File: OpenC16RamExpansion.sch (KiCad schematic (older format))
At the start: 4 parts, among them U1 74LS257, U2 74LS257, U3 4464, U4 4464

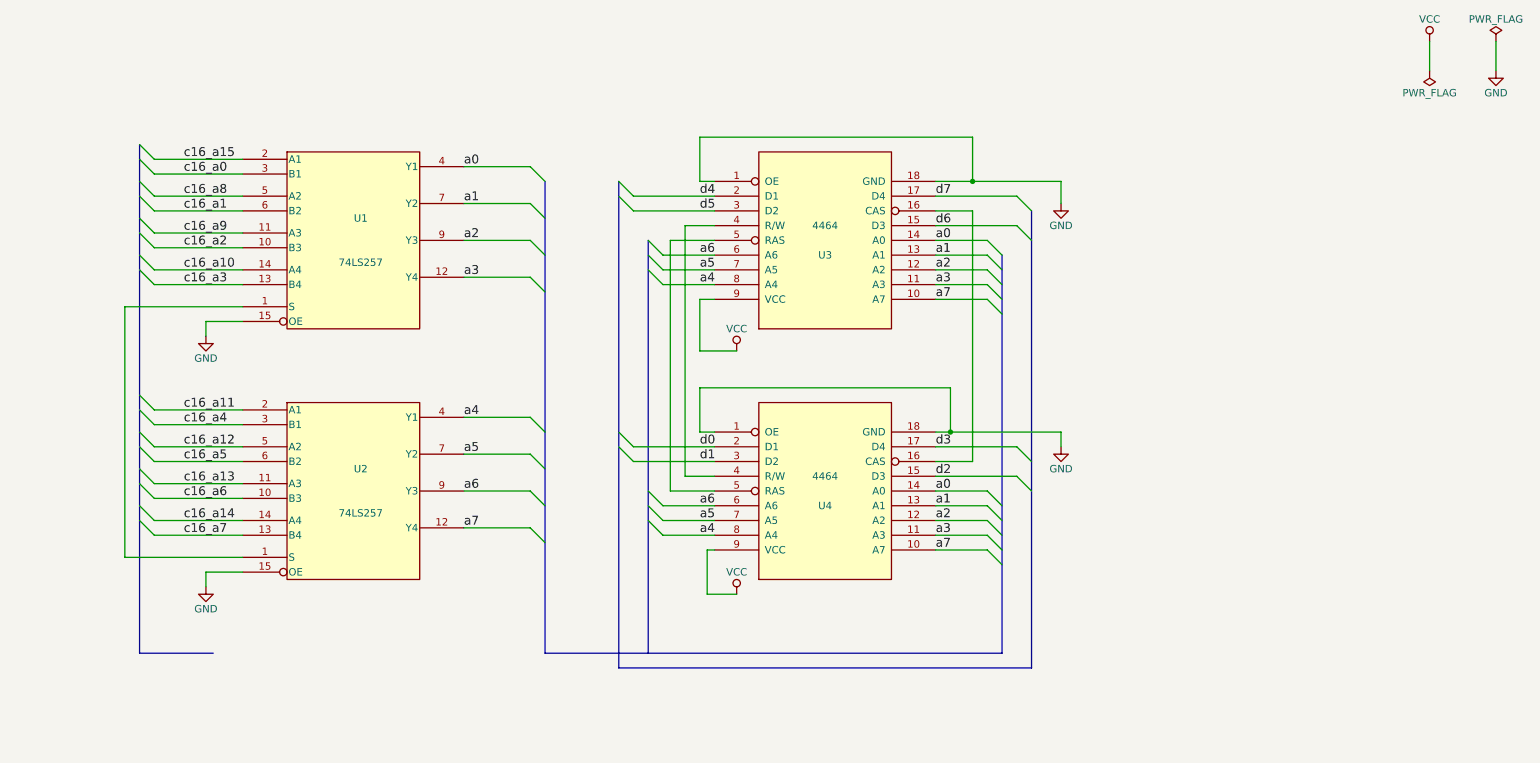
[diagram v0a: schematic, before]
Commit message: Complete schematics
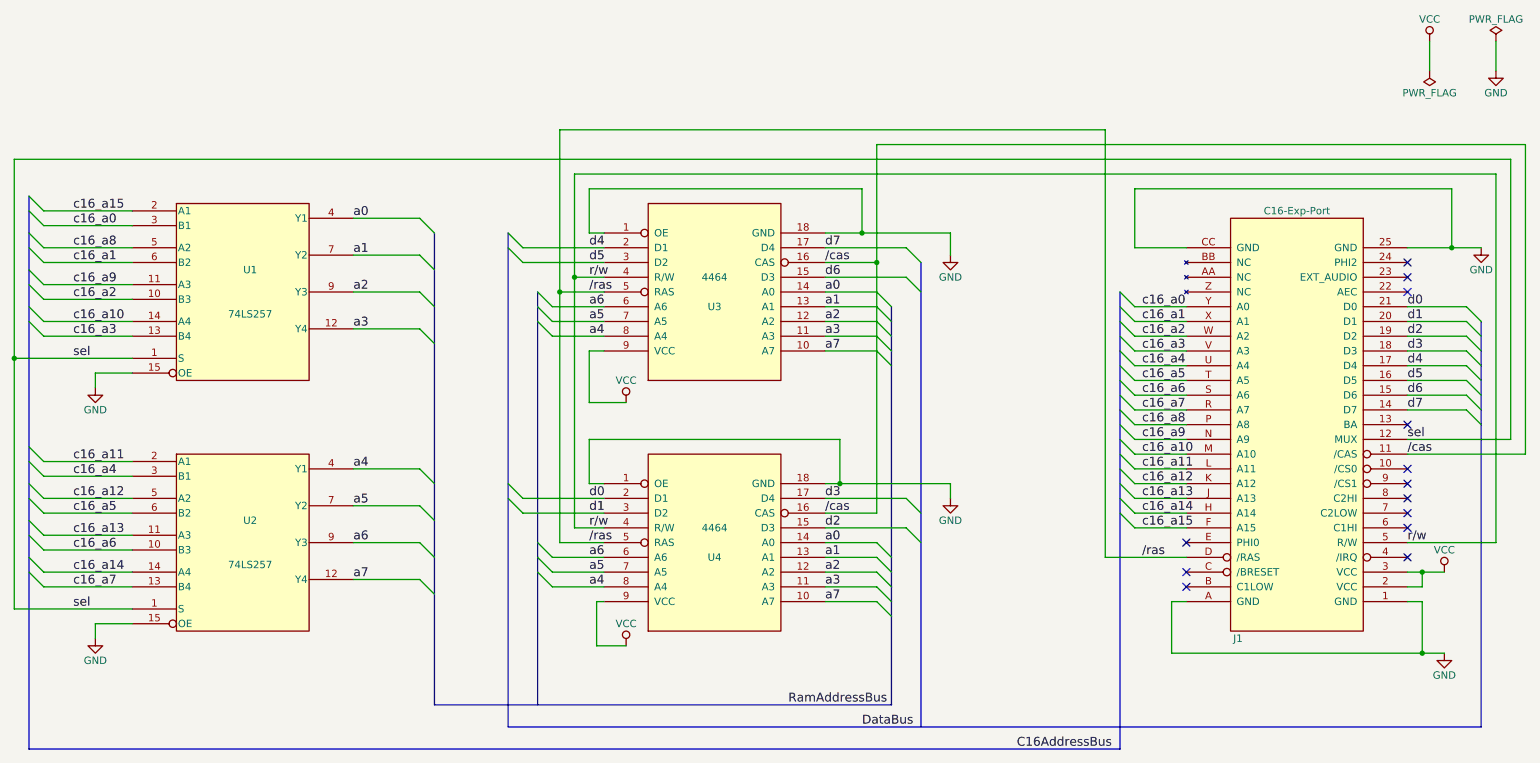
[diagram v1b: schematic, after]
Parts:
- added J1: C16-Exp-Port, C16_Cart_Conn:C16_Cart_Conn, symbol C16-Exp-Port
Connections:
- net GND: now also J1.1 (GND), J1.25 (GND), J1.A (GND), J1.CC (GND)
- net VCC: now also J1.2 (VCC), J1.3 (VCC)
- net c16_a0: now also J1.Y (A0)
- net c16_a1: now also J1.X (A1)
- net c16_a10: now also J1.M (A10)
- net c16_a11: now also J1.L (A11)
- net c16_a12: now also J1.K (A12)
- net c16_a13: now also J1.J (A13)
- net c16_a14: now also J1.H (A14)
- net c16_a15: now also J1.F (A15)
- net c16_a2: now also J1.W (A2)
- net c16_a3: now also J1.V (A3)
- net c16_a4: now also J1.U (A4)
- net c16_a5: now also J1.T (A5)
- net c16_a6: now also J1.S (A6)
- net c16_a7: now also J1.R (A7)
- net c16_a8: now also J1.P (A8)
- net c16_a9: now also J1.N (A9)
- net d0: now also J1.21 (D0)
- net d1: now also J1.20 (D1)
- net d2: now also J1.19 (D2)
- net d3: now also J1.18 (D3)
- net d4: now also J1.17 (D4)
- net d5: now also J1.16 (D5)
- net d6: now also J1.15 (D6)
- net d7: now also J1.14 (D7)
- net sel: now reaches U1.1 (S), U2.1 (S)
- net sel: now also J1.12 (MUX)
- net /cas: now reaches U3.16 (CAS), U4.16 (CAS)
- net /cas: now also J1.11 (/CAS)
- net r/w: now reaches U3.4 (R/W), U4.4 (R/W)
- net r/w: now also J1.5 (R/W)
- net /ras: now reaches U3.5 (RAS), U4.5 (RAS)
- net /ras: now also J1.D (/RAS)
- no-connect marks 0 -> 13
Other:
- moved on the sheet: U1, U2, U3, U4

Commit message: Almost there...
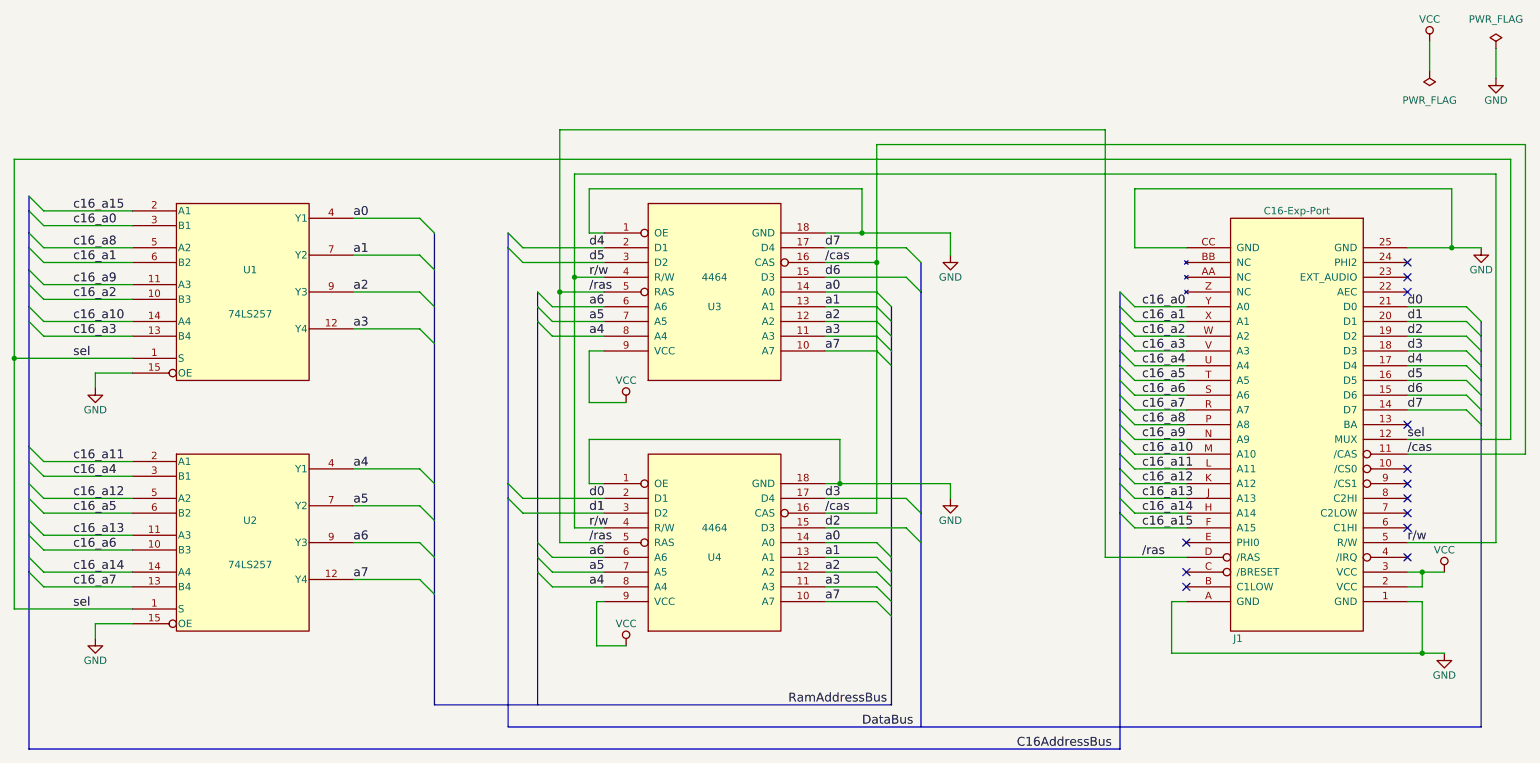
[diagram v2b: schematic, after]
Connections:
- net a0 is gone; now on net /cas: U1.4 (Y1), U3.14 (A0), U4.14 (A0)
- net a1 is gone; now on net /cas: U1.7 (Y2), U3.13 (A1), U4.13 (A1)
- net a2 is gone; now on net /cas: U1.9 (Y3), U3.12 (A2), U4.12 (A2)
- net a3 is gone; now on net /cas: U1.12 (Y4), U3.11 (A3), U4.11 (A3)
- net a7 is gone; now on net /cas: U2.12 (Y4), U3.10 (A7), U4.10 (A7)
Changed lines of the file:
@@
 L GND #PWR06
 U 1 1 598EC57B
-P 10750 1050
-F 0 "#PWR06" H 10750 800 50  0001 C CNN
-F 1 "GND" H 10750 900 50  0000 C CNN
-F 2 "" H 10750 1050 50  0001 C CNN
-F 3 "" H 10750 1050 50  0001 C CNN
-	1    10750 1050
+P 10750 1100
+F 0 "#PWR06" H 10750 850 50  0001 C CNN
+F 1 "GND" H 10750 950 50  0000 C CNN
+F 2 "" H 10750 1100 50  0001 C CNN
+F 3 "" H 10750 1100 50  0001 C CNN
+	1    10750 1100
 	1    0    0    -1
 $EndComp
@@
 L PWR_FLAG #FLG07
 U 1 1 598EC590
-P 10750 850
-F 0 "#FLG07" H 10750 925 50  0001 C CNN
-F 1 "PWR_FLAG" H 10750 1000 50  0000 C CNN
-F 2 "" H 10750 850 50  0001 C CNN
-F 3 "" H 10750 850 50  0001 C CNN
-	1    10750 850
+P 10750 900
+F 0 "#FLG07" H 10750 975 50  0001 C CNN
+F 1 "PWR_FLAG" H 10750 1100 50  0000 C CNN
+F 2 "" H 10750 900 50  0001 C CNN
+F 3 "" H 10750 900 50  0001 C CNN
+	1    10750 900
 	1    0    0    -1
 $EndComp
@@
 P 10300 1050
 F 0 "#FLG08" H 10300 1125 50  0001 C CNN
-F 1 "PWR_FLAG" H 10300 1200 50  0000 C CNN
+F 1 "PWR_FLAG" H 10300 1250 50  0000 C CNN
 F 2 "" H 10300 1050 50  0001 C CNN
 F 3 "" H 10300 1050 50  0001 C CNN
@@
 NoConn ~ 10150 4350
 Wire Wire Line
-	6200 2150 7050 2150
+	6200 2150 6450 2150
+Wire Wire Line
+	6450 2150 7050 2150
 Wire Wire Line
 	7050 2150 7050 2300
@@
 	7050 3850 7050 3950
 Wire Wire Line
-	6200 3850 7050 3850
+	6200 3850 6300 3850
+Wire Wire Line
+	6300 3850 7050 3850
 Wire Wire Line
 	4850 4950 4650 4950
@@
 	10300 850  10300 1050
 Wire Wire Line
-	10750 1050 10750 850
+	10750 1100 10750 900
 Wire Wire Line
 	6550 4050 6200 4050
 Wire Wire Line
-	6550 1550 6550 4050
+	6550 1550 6550 2350
+Wire Wire Line
+	6550 2350 6550 2550
+Wire Wire Line
+	6550 2550 6550 2650
+Wire Wire Line
+	6550 2650 6550 2750
+Wire Wire Line
+	6550 2750 6550 2850
+Wire Wire Line
+	6550 2850 6550 2950
+Wire Wire Line
+	6550 2950 6550 4050
 Wire Wire Line
 	6550 2350 6200 2350
@@
 	6200 4650 6550 4650
 Wire Bus Line
-	6650 2650 6650 5350
+	6650 2650 6650 2750
+Wire Bus Line
+	6650 2750 6650 2850
+Wire Bus Line
+	6650 2850 6650 2950
+Wire Bus Line
+	6650 2950 6650 3050
+Wire Bus Line
+	6650 3050 6650 4350
+Wire Bus Line
+	6650 4350 6650 4450
+Wire Bus Line
+	6650 4450 6650 4550
+Wire Bus Line
+	6650 4550 6650 4650
+Wire Bus Line
+	6650 4650 6650 4750
+Wire Bus Line
+	6650 4750 6650 5350
 Wire Wire Line
 	4400 4250 4700 4250
 Wire Wire Line
-	4400 1450 4400 4250
+	4400 1450 4400 2550
+Wire Wire Line
+	4400 2550 4400 4250
 Wire Wire Line
 	4400 2550 4700 2550
@@
 	4700 4550 4350 4550
 Wire Bus Line
-	4250 2550 4250 5350
+	4250 2550 4250 2650
+Wire Bus Line
+	4250 2650 4250 2750
+Wire Bus Line
+	4250 2750 4250 4250
+Wire Bus Line
+	4250 4250 4250 4350
+Wire Bus Line
+	4250 4350 4250 4450
+Wire Bus Line
+	4250 4450 4250 5350
 Wire Wire Line
 	1500 3100 1250 3100
@@
 	1500 3000 700  3000
 Wire Wire Line
-	700  1650 700  4700
+	700  1650 700  3000
+Wire Wire Line
+	700  3000 700  4700
 Wire Wire Line
 	700  4700 1500 4700
@@
 	6200 4150 6750 4150
 Wire Bus Line
-	6850 2350 6850 5500
+	6850 2350 6850 2550
+Wire Bus Line
+	6850 2550 6850 4050
+Wire Bus Line
+	6850 4050 6850 4250
+Wire Bus Line
+	6850 4250 6850 5500
 Wire Bus Line
 	10650 5500 4050 5500
@@
 	4700 4050 4150 4050
 Wire Bus Line
-	4050 5500 4050 2150
+	4050 5500 4050 3950
+Wire Bus Line
+	4050 3950 4050 3850
+Wire Bus Line
+	4050 3850 4050 2250
+Wire Bus Line
+	4050 2250 4050 2150
 Wire Wire Line
 	4500 4150 4700 4150
 Wire Wire Line
-	4500 1750 4500 4150
+	4500 1750 4500 2450
+Wire Wire Line
+	4500 2450 4500 4150
 Wire Wire Line
 	4500 2450 4700 2450
@@
 	1500 4550 900  4550
 Wire Bus Line
-	800  1900 800  5650
+	800  1900 800  2000
+Wire Bus Line
+	800  2000 800  2150
+Wire Bus Line
+	800  2150 800  2250
+Wire Bus Line
+	800  2250 800  2400
+Wire Bus Line
+	800  2400 800  2500
+Wire Bus Line
+	800  2500 800  2650
+Wire Bus Line
+	800  2650 800  2750
+Wire Bus Line
+	800  2750 800  3600
+Wire Bus Line
+	800  3600 800  3700
+Wire Bus Line
+	800  3700 800  3850
+Wire Bus Line
+	800  3850 800  3950
+Wire Bus Line
+	800  3950 800  4100
+Wire Bus Line
+	800  4100 800  4200
+Wire Bus Line
+	800  4200 800  4350
+Wire Bus Line
+	800  4350 800  4450
+Wire Bus Line
+	800  4450 800  5650
 Wire Wire Line
 	3000 2050 3450 2050
@@
 	3000 4500 3450 4500
 Wire Bus Line
-	3550 2150 3550 5350
+	3550 2150 3550 2400
+Wire Bus Line
+	3550 2400 3550 2650
+Wire Bus Line
+	3550 2650 3550 2900
+Wire Bus Line
+	3550 2900 3550 3850
+Wire Bus Line
+	3550 3850 3550 4100
+Wire Bus Line
+	3550 4100 3550 4350
+Wire Bus Line
+	3550 4350 3550 4600
+Wire Bus Line
+	3550 4600 3550 5350
 Wire Wire Line
 	8650 2650 8300 2650
@@
 	8650 4150 8300 4150
 Wire Bus Line
-	8200 2550 8200 5650
+	8200 2550 8200 2650
+Wire Bus Line
+	8200 2650 8200 2750
+Wire Bus Line
+	8200 2750 8200 2850
+Wire Bus Line
+	8200 2850 8200 2950
+Wire Bus Line
+	8200 2950 8200 3050
+Wire Bus Line
+	8200 3050 8200 3150
+Wire Bus Line
+	8200 3150 8200 3250
+Wire Bus Line
+	8200 3250 8200 3350
+Wire Bus Line
+	8200 3350 8200 3450
+Wire Bus Line
+	8200 3450 8200 3550
+Wire Bus Line
+	8200 3550 8200 3650
+Wire Bus Line
+	8200 3650 8200 3750
+Wire Bus Line
+	8200 3750 8200 3850
+Wire Bus Line
+	8200 3850 8200 3950
+Wire Bus Line
+	8200 3950 8200 4050
+Wire Bus Line
+	8200 4050 8200 5650
 Wire Wire Line
 	8650 2250 8300 2250
@@
 	10450 1850 10450 2250
 Wire Wire Line
-	10150 2250 10650 2250
+	10150 2250 10450 2250
+Wire Wire Line
+	10450 2250 10650 2250
 Connection ~ 10450 2250
 Wire Wire Line
@@
 	8550 4650 8550 5000
 Wire Wire Line
-	8550 5000 10400 5000
+	8550 5000 10250 5000
+Wire Wire Line
+	10250 5000 10400 5000
 Wire Wire Line
 	10250 5000 10250 4650
@@
 	10150 3350 10550 3350
 Wire Bus Line
-	10650 2750 10650 5500
+	10650 2750 10650 2850
+Wire Bus Line
+	10650 2850 10650 2950
+Wire Bus Line
+	10650 2950 10650 3050
+Wire Bus Line
+	10650 3050 10650 3150
+Wire Bus Line
+	10650 3150 10650 3250
+Wire Bus Line
+	10650 3250 10650 3350
+Wire Bus Line
+	10650 3350 10650 3450
+Wire Bus Line
+	10650 3450 10650 5500
 Wire Bus Line
 	3550 5350 6650 5350
@@
 $EndComp
 Wire Wire Line
-	10150 4450 10400 4450
+	10150 4450 10250 4450
+Wire Wire Line
+	10250 4450 10400 4450
 Wire Wire Line
 	10150 4550 10250 4550
